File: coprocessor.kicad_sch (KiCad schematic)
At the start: 2 parts

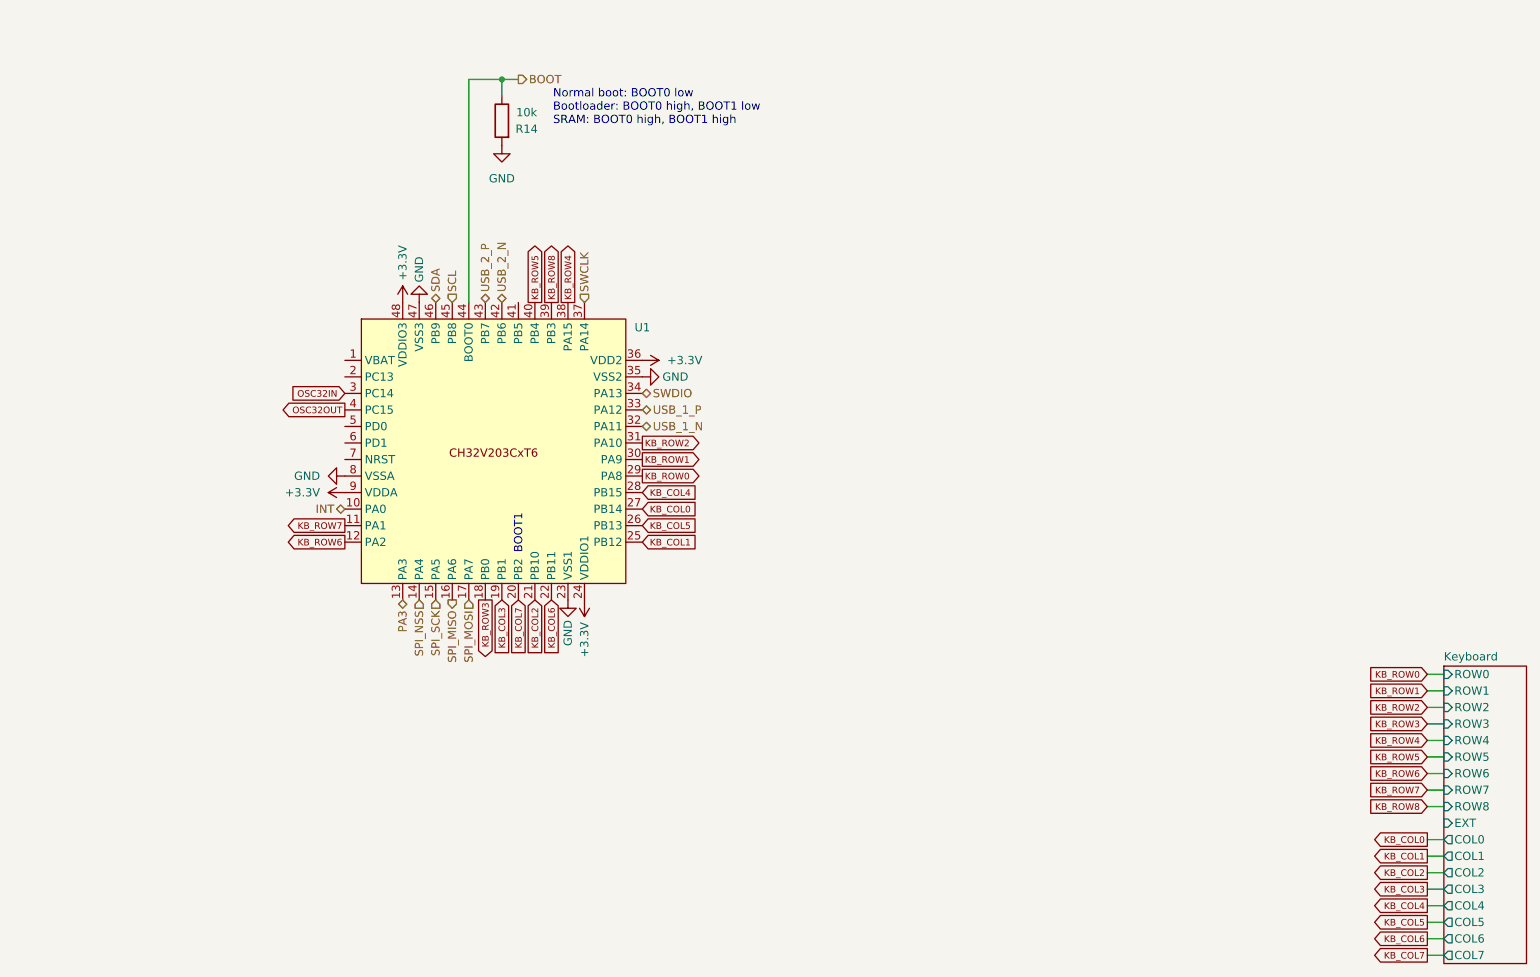
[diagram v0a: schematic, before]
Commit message: Work in progress
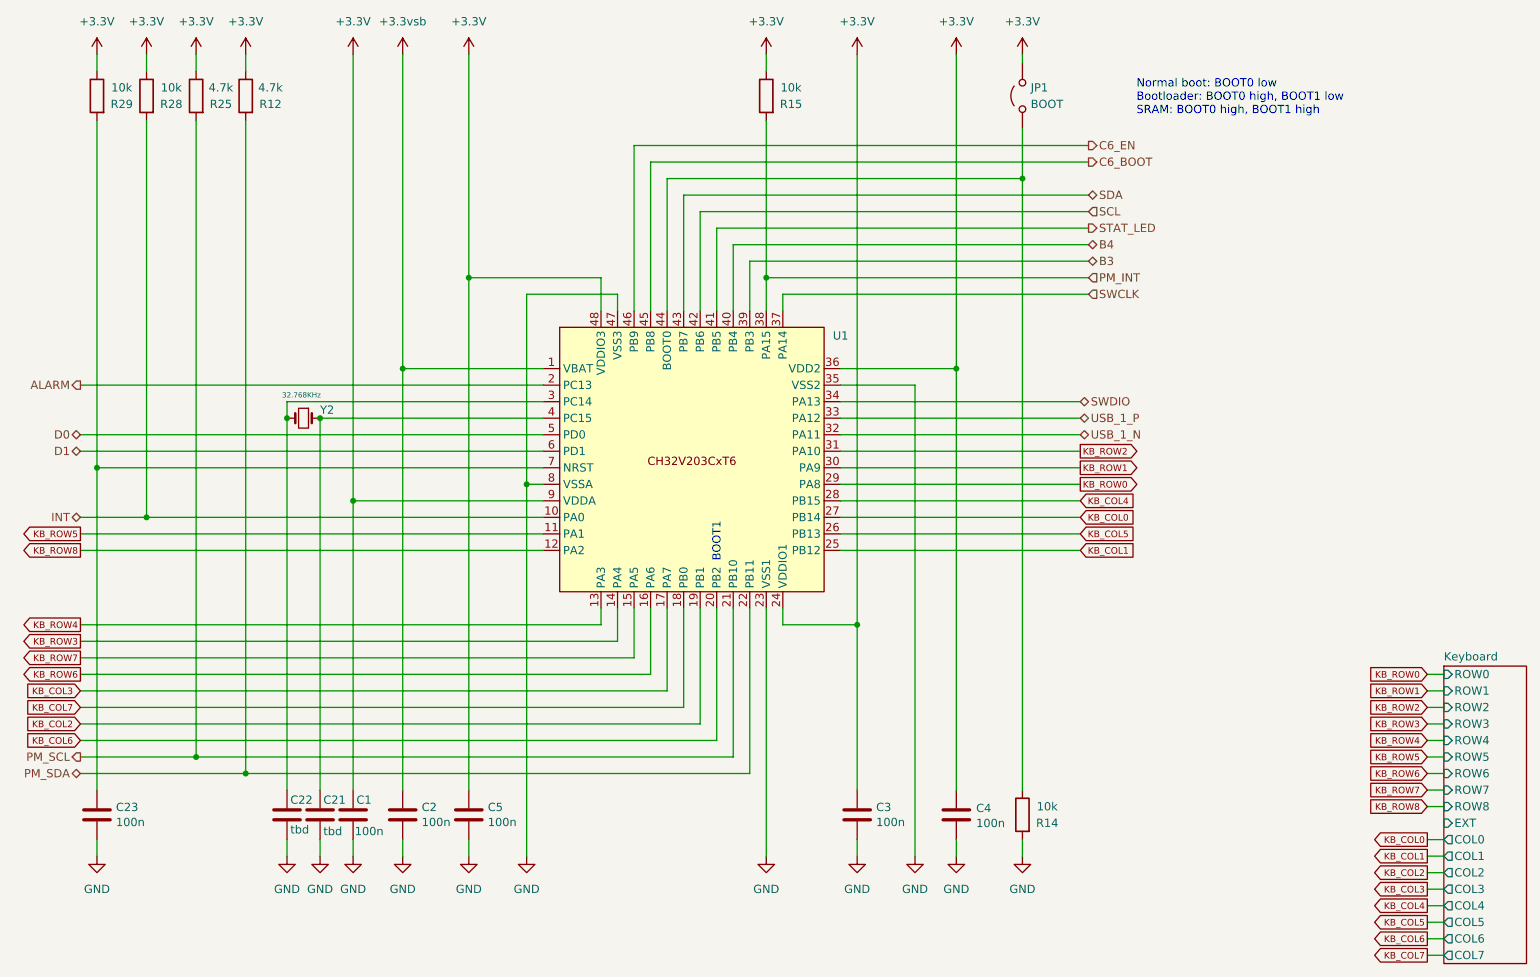
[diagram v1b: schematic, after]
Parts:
- added C1, C2, C23, C3, C4, C5: 100n, Capacitor_SMD:C_0402_1005Metric, symbol symbols:C
- added C21, C22: tbd, symbol Device:C
- added JP1: BOOT, Jumper:SolderJumper-2_P1.3mm_Open_RoundedPad1.0x1.5mm, symbol Jumper:Jumper_2_Open
- added R12, R25: 4.7k, Resistor_SMD:R_0402_1005Metric, symbol symbols:R
- added R15, R28, R29: 10k, Resistor_SMD:R_0402_1005Metric, symbol symbols:R
- added Y2: 32.768KHz, Crystal:Crystal_SMD_3215-2Pin_3.2x1.5mm, symbol symbols:Crystal_Small
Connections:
- net PA3 is gone; now on net KB_ROW4: U1.13 (PA3)
- net SPI_MISO is gone; now on net KB_ROW6: U1.16 (PA6)
- net SPI_MOSI is gone; now on net KB_COL3: U1.17 (PA7)
- net SPI_NSS is gone; now on net KB_ROW3: U1.14 (PA4)
- net SPI_SCK is gone; now on net KB_ROW7: U1.15 (PA5)
- net USB_2_N is gone; now on net SCL: U1.42 (PB6)
- net USB_2_P is gone; now on net SDA: U1.43 (PB7)
- net +3.3V: now also C1.1, C3.1, C4.1, C5.1, JP1.2 (B), R12.1, R15.1, R25.1, R28.1, R29.1
- net GND: now also C1.2, C2.2, C21.2, C22.2, C23.2, C3.2, C4.2, C5.2
- net INT: now also R28.2
- net KB_COL2: now also U1.19 (PB1); no longer U1.21 (PB10)
- net KB_COL3: no longer U1.19 (PB1)
- net KB_COL6: now also U1.20 (PB2); no longer U1.22 (PB11)
- net KB_COL7: now also U1.18 (PB0); no longer U1.20 (PB2)
- net KB_ROW3: no longer U1.18 (PB0)
- net KB_ROW4: no longer U1.38 (PA15)
- net KB_ROW5: now also U1.11 (PA1); no longer U1.40 (PB4)
- net KB_ROW6: no longer U1.12 (PA2)
- net KB_ROW7: no longer U1.11 (PA1)
- net KB_ROW8: now also U1.12 (PA2); no longer U1.39 (PB3)
- net SCL: no longer U1.45 (PB8)
- net SDA: no longer U1.46 (PB9)
- net +3.3vsb: now reaches U1.1 (VBAT)
- net +3.3vsb: now also C2.1
- net ALARM: now reaches U1.2 (PC13)
- net STAT_LED: now reaches U1.41 (PB5)
- net D0: now reaches U1.5 (PD0)
- net D1: now reaches U1.6 (PD1)
- net at U1.7 (NRST): now also C23.1, R29.2
- net BOOT: no longer names the net of R14.1, U1.44 (BOOT0)
- net BOOT: now also JP1.1 (A)
- net OSC32IN: no longer names the net of U1.3 (PC14)
- net OSC32IN: now also C22.1, Y2.2
- net OSC32OUT: no longer names the net of U1.4 (PC15)
- net OSC32OUT: now also C21.1, Y2.1
- new net B3: U1.39 (PB3)
- new net B4: U1.40 (PB4)
- new net C6_BOOT: U1.45 (PB8)
- new net C6_EN: U1.46 (PB9)
- new net PM_INT: R15.2, U1.38 (PA15)
- new net PM_SCL: R25.2, U1.21 (PB10)
- new net PM_SDA: R12.2, U1.22 (PB11)
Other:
- moved on the sheet: R14, U1
